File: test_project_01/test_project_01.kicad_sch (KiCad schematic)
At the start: 3 parts, among them J7 USB_B_Mini, J8 Micro_SD_Card_Det

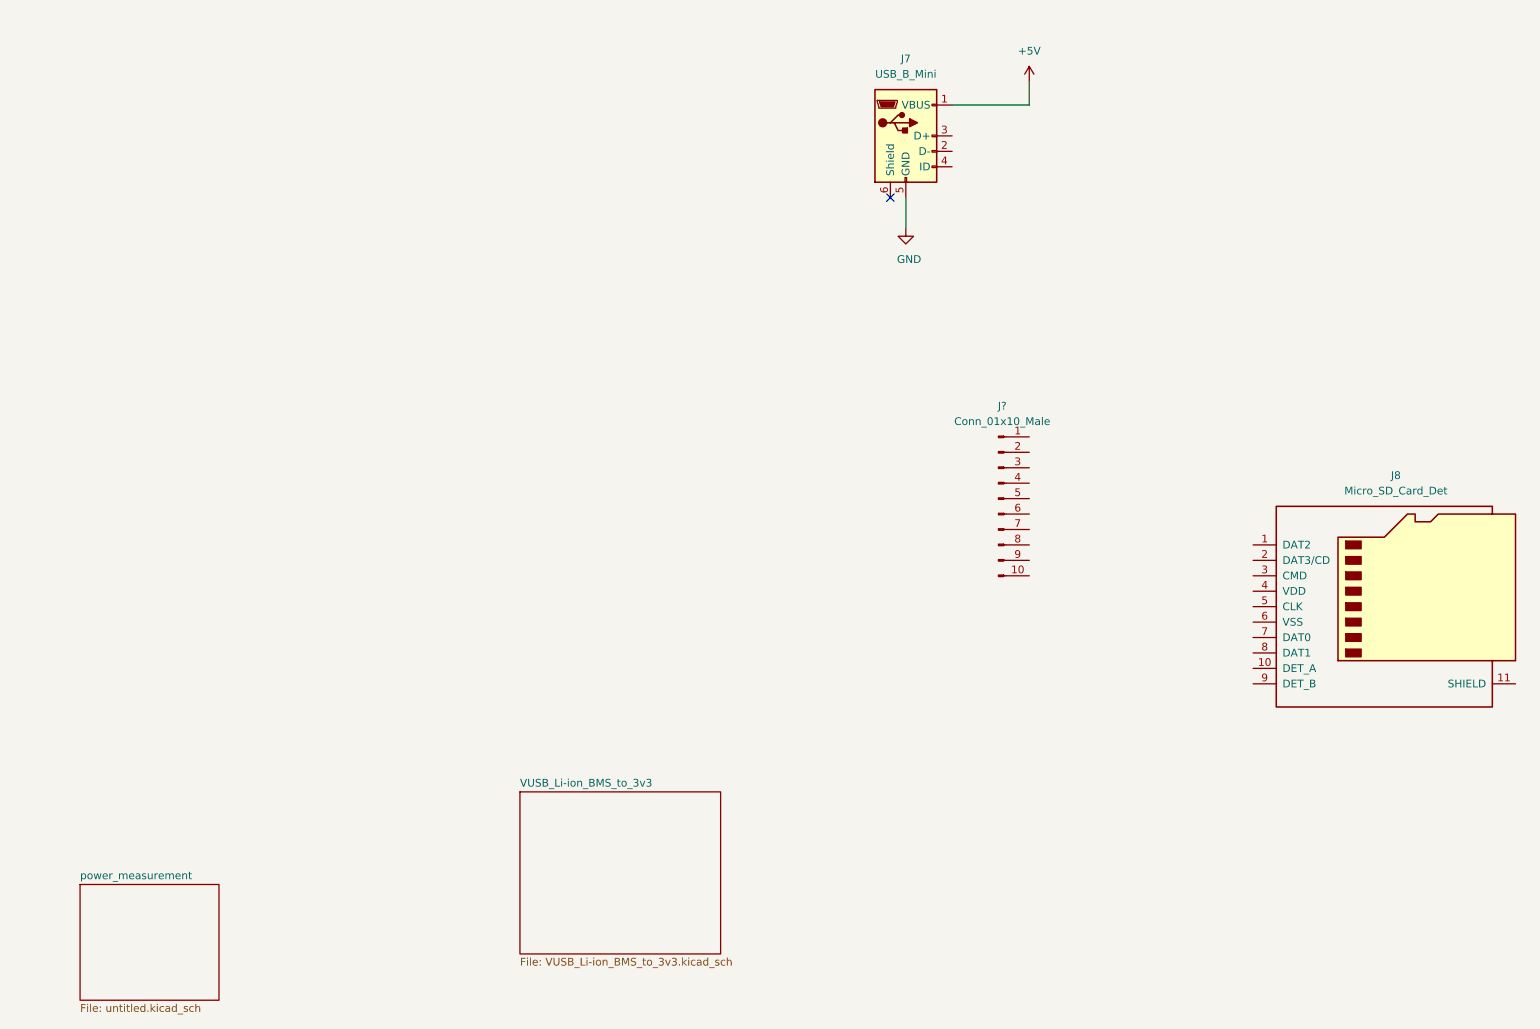
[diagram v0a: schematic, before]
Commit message: v
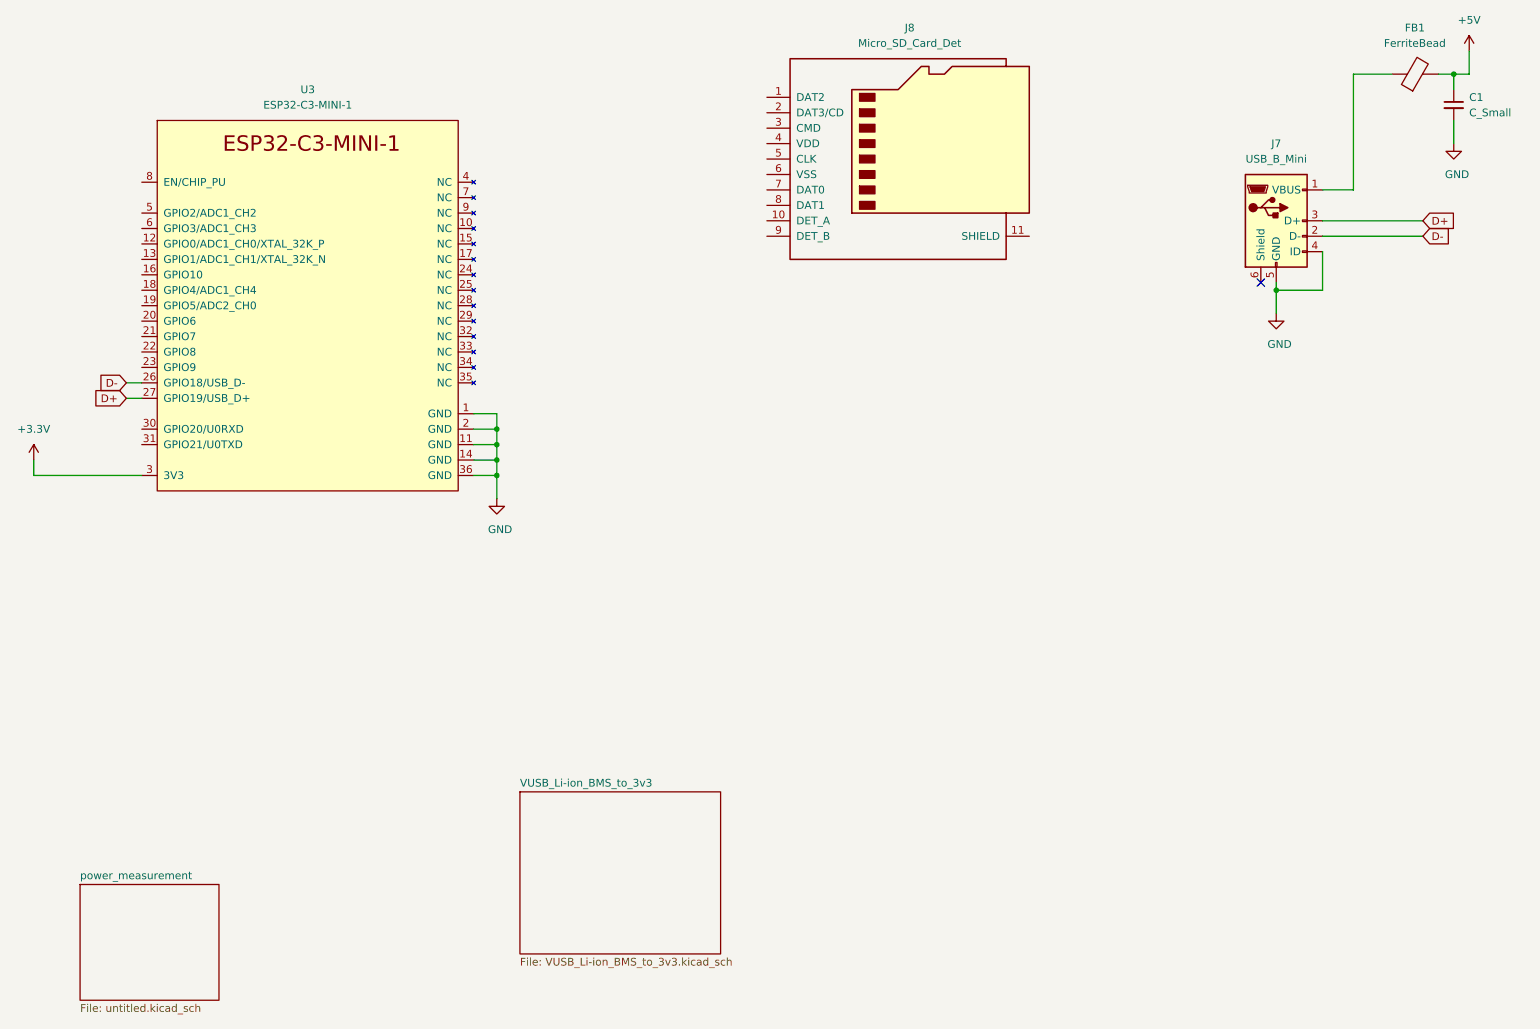
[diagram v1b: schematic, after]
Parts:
- removed J?: Conn_01x10_Male, symbol Connector:Conn_01x10_Male
- added C1: C_Small, symbol Device:C_Small
- added FB1: FerriteBead, symbol Device:FerriteBead
- added U3: ESP32-C3-MINI-1, Espressif:ESP32-C3-MINI-1_Hand-Soldering, symbol Espressif:ESP32-C3-MINI-1
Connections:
- net +5V: now also C1.1, FB1.2; no longer J7.1 (VBUS)
- net GND: now also J7.4 (ID), C1.2, U3.1 (GND), U3.11 (GND), U3.14 (GND), U3.2 (GND), U3.36 (GND)
- net D-: now reaches J7.2 (D-)
- net D-: now also U3.26 (GPIO18/USB_D-)
- net D+: now reaches J7.3 (D+)
- net D+: now also U3.27 (GPIO19/USB_D+)
- new net: FB1.1, J7.1 (VBUS)
- new net +3V3: U3.3 (3V3)
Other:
- moved on the sheet: J7, J8
